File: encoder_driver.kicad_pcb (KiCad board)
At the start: 2 copper layers, 75.1 x 55.9 mm, 23 parts, among them J1 Conn_01x06_Male, J2 Conn_01x06_Male, J3 Conn_01x06, J4 Conn_01x02_Male, Q1 Si2319CDS, U1 TLE5012B, U2 ISO7321C, U3 ISO7320C, U4 B0505T-1W

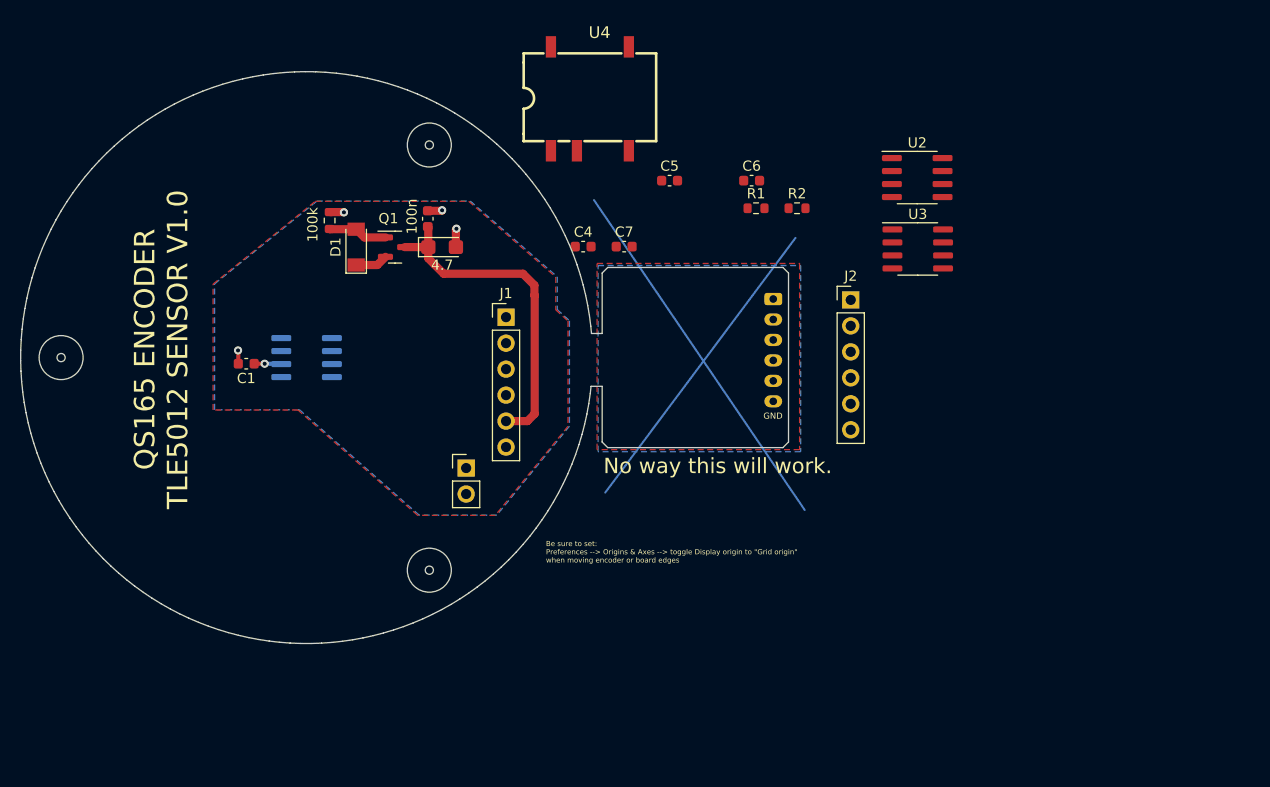
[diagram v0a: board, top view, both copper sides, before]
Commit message: near final draft
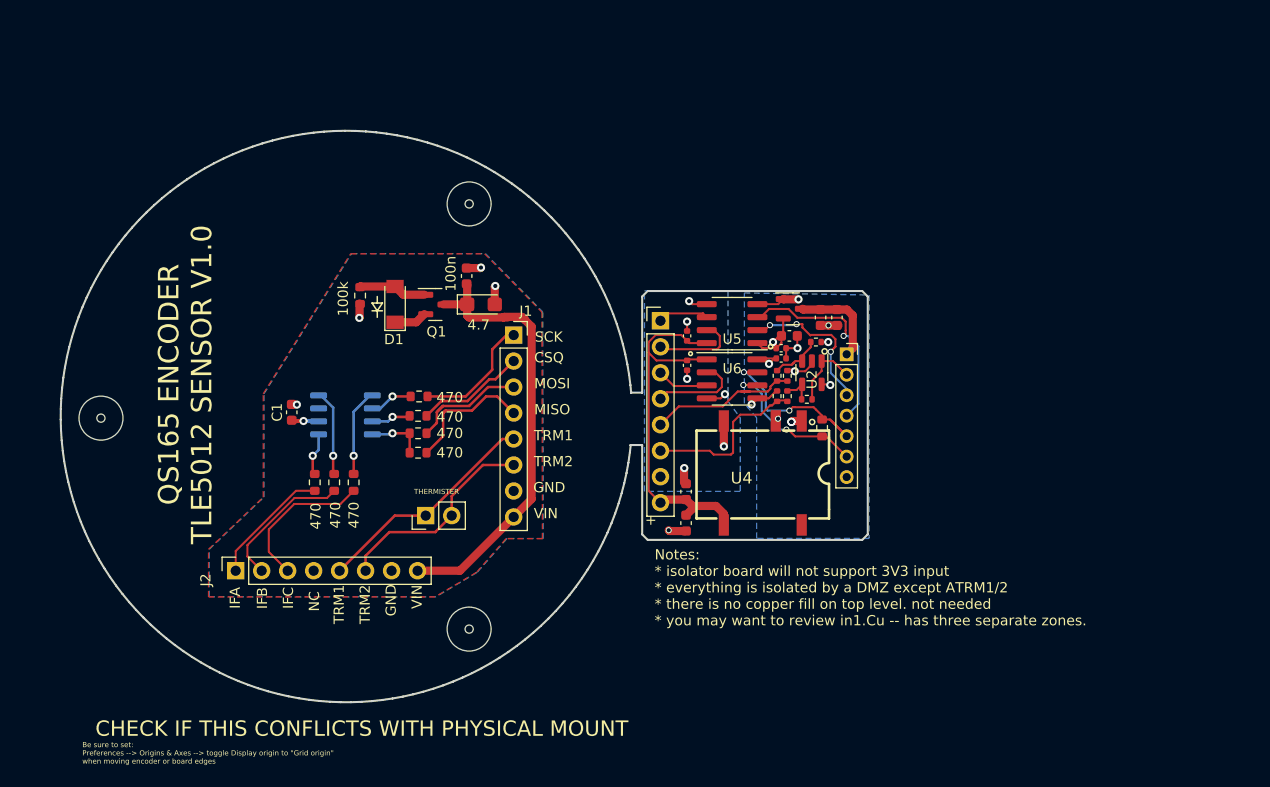
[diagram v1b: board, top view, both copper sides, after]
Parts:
- removed C4, C7: 100n, Capacitor_SMD:C_0603_1608Metric
- removed the J3 at (147.2, 70.5)
- removed the REF** at (113.6, 97.0)
- removed the REF** at (113.6, 55.4)
- removed the REF** at (77.6, 76.2)
- added C10: 1uF, Capacitor_SMD:C_0603_1608Metric, F.Cu at (138.7, 89.3)
- added C11: 100n, Capacitor_SMD:C_0402_1005Metric, F.Cu at (148.0, 76.3)
- added C15: 1uF, Capacitor_SMD:C_0603_1608Metric, F.Cu at (153.4, 72.3)
- added C16: 1uF, Capacitor_SMD:C_0603_1608Metric, F.Cu at (148.8, 74.1)
- added C17: 1uF, Capacitor_SMD:C_0603_1608Metric, F.Cu at (151.8, 72.3)
- added C8: 100n, Capacitor_SMD:C_0402_1005Metric, F.Cu at (148.0, 75.3)
- added C9: 1uF, Capacitor_SMD:C_0603_1608Metric, F.Cu at (138.7, 92.4)
- added J4: Conn_01x07, Connector_PinSocket_2.00mm:PinSocket_1x07_P2.00mm_Vertical, F.Cu at (154.4, 75.9)
- added J5: Conn_01x08_Female, Connector_PinHeader_2.54mm:PinHeader_1x08_P2.54mm_Vertical, F.Cu at (136.2, 72.6)
- added R10: 100k, Resistor_SMD:R_0402_1005Metric, F.Cu at (151.4, 74.7)
- added R11: 100k, Resistor_SMD:R_0402_1005Metric, F.Cu at (148.6, 80.0)
- added R12: 100k, Resistor_SMD:R_0402_1005Metric, F.Cu at (150.5, 80.3)
- added R13: 4.7k, Resistor_SMD:R_0402_1005Metric, F.Cu at (147.6, 80.0)
- added R14: 100k, Resistor_SMD:R_0402_1005Metric, F.Cu at (147.6, 78.0)
- added R15: 470, Resistor_SMD:R_0603_1608Metric, F.Cu at (152.0, 83.1)
- added R3: 470, Resistor_SMD:R_0603_1608Metric, F.Cu at (106.2, 88.4)
- added R4: 470, Resistor_SMD:R_0603_1608Metric, F.Cu at (112.6, 80.0)
- added R5: 470, Resistor_SMD:R_0603_1608Metric, F.Cu at (112.5, 81.9)
- added R6: 470, Resistor_SMD:R_0603_1608Metric, F.Cu at (112.5, 83.6)
- added R7: 470, Resistor_SMD:R_0603_1608Metric, F.Cu at (112.5, 85.5)
- added R9: 4.7k, Resistor_SMD:R_0402_1005Metric, F.Cu at (148.6, 78.0)
- added REF**: MountingHole_4.3mm_M4, MountingHole:MountingHole_4.3mm_M4, F.Cu at (117.5, 102.7)
- added REF**: MountingHole_4.3mm_M4, MountingHole:MountingHole_4.3mm_M4, F.Cu at (117.5, 61.2)
- added REF**: MountingHole_4.3mm_M4, MountingHole:MountingHole_4.3mm_M4, F.Cu at (81.5, 82.1)
- added U5: CA-IS3720, Package_SO:SOIC-8_3.9x4.9mm_P1.27mm, F.Cu at (143.2, 72.9)
- added U6: CA-IS3721C, Package_SO:SOIC-8_3.9x4.9mm_P1.27mm, F.Cu at (143.2, 78.3)
- C5, C6: footprint Capacitor_SMD:C_0603_1608Metric -> Capacitor_SMD:C_0402_1005Metric
- D1: value BZV55B10 -> BZV55C6V2
- J1, J2: value Conn_01x06_Male -> Conn_01x08_Female; footprint Connector_PinHeader_2.54mm:PinHeader_1x06_P2.54mm_Vertical -> Connector_PinSocket_2.54mm:PinSocket_1x08_P2.54mm_Vertical
- R1, R2: value 10k -> 470
- U1: value TLE5012B -> TLE5012b; footprint Package_SO:SOIC-8_3.9x4.9mm_P1.27mm -> Package_SO:my_Infineon_PG-DSO-8
- U2: value ISO7321C -> MCP6L01Rx-xOT; footprint Package_SO:SOIC-8_3.9x4.9mm_P1.27mm -> Package_TO_SOT_SMD:SOT-23-5
- U3: value ISO7320C -> XC6206PxxxMR; footprint Package_SO:SOIC-8_3.9x4.9mm_P1.27mm -> Package_TO_SOT_SMD:SOT-23
- moved J2 65.7 mm to (94.7, 97.0), turned to 90 degrees
- moved R2 52.6 mm to (104.3, 88.4), turned to -90 degrees
- moved R1 50.8 mm to (102.4, 88.4), turned to -90 degrees
- moved U4 40.3 mm to (146.2, 87.5), turned to 180 degrees
- moved U2 21.7 mm to (151.0, 77.7), turned to -90 degrees
- moved C6 19.1 mm to (138.8, 77.0), turned to -90 degrees
- moved C5 15.3 mm to (138.8, 74.1), turned to 90 degrees
- moved U3 13.5 mm to (149.1, 71.4)
- moved R8 7.92 mm to (106.8, 70.1), turned to -90 degrees
- moved Q1 6.86 mm to (114.2, 71.0)
- moved C3 6.77 mm to (118.7, 71.0)
- moved U1 6.77 mm to (105.4, 81.8)
- moved C2 6.77 mm to (117.2, 68.2)
- moved D1 6.77 mm to (110.2, 71.0)
- moved C1 6.51 mm to (100.2, 81.5), turned to 90 degrees
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- renumbered J4 to J3, R3 to R8
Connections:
- C5 pad 1: _+5 -> A+5V
- C5 pad 2: _GND -> AGND
- C6 pad 1: _+5 -> A+5V
- C6 pad 2: _GND -> AGND
- J1 pad 1: unconnected-(J1-Pad1) -> SCK
- J1 pad 2: unconnected-(J1-Pad2) -> CSQ
- J1 pad 3: unconnected-(J1-Pad3) -> MOSI
- J1 pad 4: TEMP -> MISO
- J1 pad 5: VIN -> TRM1
- J1 pad 6: GND -> TRM2
- J2 pad 1: unconnected-(J2-Pad1) -> IFA
- J2 pad 2: unconnected-(J2-Pad2) -> IFB
- J2 pad 3: unconnected-(J2-Pad3) -> IFC
- J2 pad 4: _TEMP -> unconnected-(J2-Pad4)
- J2 pad 5: _+5 -> TRM1
- J2 pad 6: _GND -> TRM2
- J3 pad 1: unconnected-(J4-Pad1) -> TRM1
- J3 pad 2: GND -> TRM2
- R1 pad 1: unconnected-(R1-Pad1) -> Net-(R1-Pad1)
- R1 pad 2: unconnected-(R1-Pad2) -> IFA
- R2 pad 1: unconnected-(R2-Pad1) -> Net-(R2-Pad1)
- R2 pad 2: unconnected-(R2-Pad2) -> IFB
- U1 pad 1: unconnected-(U1-Pad1) -> Net-(R3-Pad1)
- U1 pad 2: unconnected-(U1-Pad2) -> Net-(R4-Pad2)
- U1 pad 3: unconnected-(U1-Pad3) -> Net-(R5-Pad2)
- U1 pad 4: unconnected-(U1-Pad4) -> Net-(R6-Pad2)
- U1 pad 5: unconnected-(U1-Pad5) -> Net-(R1-Pad1)
- U1 pad 8: unconnected-(U1-Pad8) -> Net-(R2-Pad1)
- U2 pad 1: unconnected-(U2-Pad1) -> BTEMP
- U2 pad 2: unconnected-(U2-Pad2) -> +3V3
- U2 pad 3: unconnected-(U2-Pad3) -> Net-(R10-Pad1)
- U2 pad 4: unconnected-(U2-Pad4) -> Net-(R11-Pad1)
- U2 pad 5: unconnected-(U2-Pad5) -> BGND
- U3 pad 1: unconnected-(U3-Pad1) -> BGND
- U3 pad 2: unconnected-(U3-Pad2) -> +3V3
- U3 pad 3: unconnected-(U3-Pad3) -> B+5V
- U4 pad 1: unconnected-(U4-Pad1) -> BGND
- U4 pad 2: unconnected-(U4-Pad2) -> B+5V
- U4 pad 3: unconnected-(U4-Pad3) -> AGND
- U4 pad 4: unconnected-(U4-Pad4) -> A+5V
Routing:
- net A+5V: track 0.00 -> 37.7 mm
- net TRM1: track 0.00 -> 22.4 mm
- net TRM2: track 0.00 -> 20.7 mm
- net BSCLK: track 0.00 -> 20.1 mm, vias 0 -> 1
- net B+5V: track 0.00 -> 19.1 mm, vias 0 -> 1
- net BMISO: track 0.00 -> 17.6 mm, vias 0 -> 2
- net ATRM2: track 0.00 -> 17.0 mm
- net BCSQ: track 0.00 -> 15.4 mm, vias 0 -> 3
- net BMOSI: track 0.00 -> 15.4 mm, vias 0 -> 2
- net ATRM1: track 0.00 -> 15.2 mm
- net BGND: track 0.00 -> 14.9 mm, vias 0 -> 8
- net IFC: track 0.00 -> 14.8 mm
- net IFB: track 0.00 -> 13.8 mm
- net MISO: track 0.00 -> 13.1 mm
- net +3V3: track 0.00 -> 12.9 mm, vias 0 -> 3
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- added copper zone on In1.Cu, net +3V3
- added copper zone on B.Cu, net AGND
- added copper zone on In1.Cu, net AGND
- added copper zone on In2.Cu, net AGND
- added copper zone on B.Cu, net BGND
- added copper zone on In1.Cu, net BGND
- added copper zone on In2.Cu, net BGND
- added copper zone on In1.Cu, net GND
- added copper zone on In2.Cu, net GND
- removed copper zone on F.Cu, net _+5
- removed copper zone on B.Cu, net _GND
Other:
- board size 75.1 x 55.9 mm -> 78.9 x 55.9 mm
- copper layers 2 -> 4
- board text added: "+"
- board text added: "CHECK IF THIS CONFLICTS WITH PHYSICAL MOUNT"
- board text added: "CLK"
- board text added: "CSQ"
- board text added: "IFA"
- board text added: "IFB"
- board text added: "IFC"
- board text added: "MISO"
- board text added: "MOSI"
- board text added: "NC"
- board text added: "Notes: * isolator board will not support 3V3 input * everything is isolated by a DMZ except ATRM1/2 * there is no copper fill on top level. not needed * you may want to review in1.Cu -- has three separate zones."
- board text added: "SCK"
- board text added: "SSC Isolator V1.0"
- board text added: "TEMP"
- board text added: "THERMISTER"
- board text added: "TRM1"
- board text added: "TRM2"
- board text added: "VIN"
- board text added: "VOUT"
- board text added: "V_IN"
- board text removed: "+5"
- board text removed: "A"
- board text removed: "A- A+ B- B+ C- C+ T2 T2 VN GD"
- board text removed: "B"
- board text removed: "I"
- board text removed: "No way this will work."
- board text removed: "T"
- board text removed: "VN GD T1 T2 I+ I- B+ B- A+ A-"
